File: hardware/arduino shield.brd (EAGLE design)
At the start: 100 x 54.6 mm, 26 parts, among them U1 ADS1115IDGST, U2 ARDUINO-MEGAPRO-5V, X4 MSTBA4

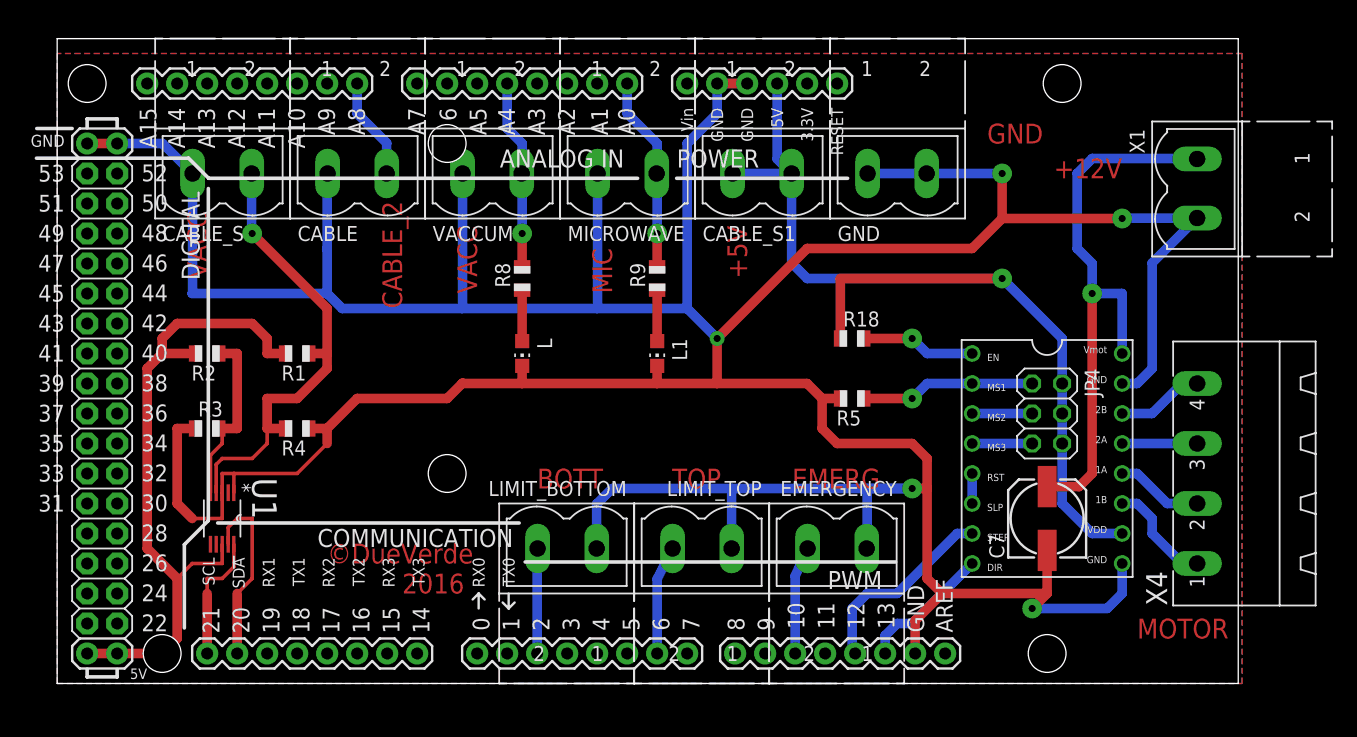
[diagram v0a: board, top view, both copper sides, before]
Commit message: hardware changes
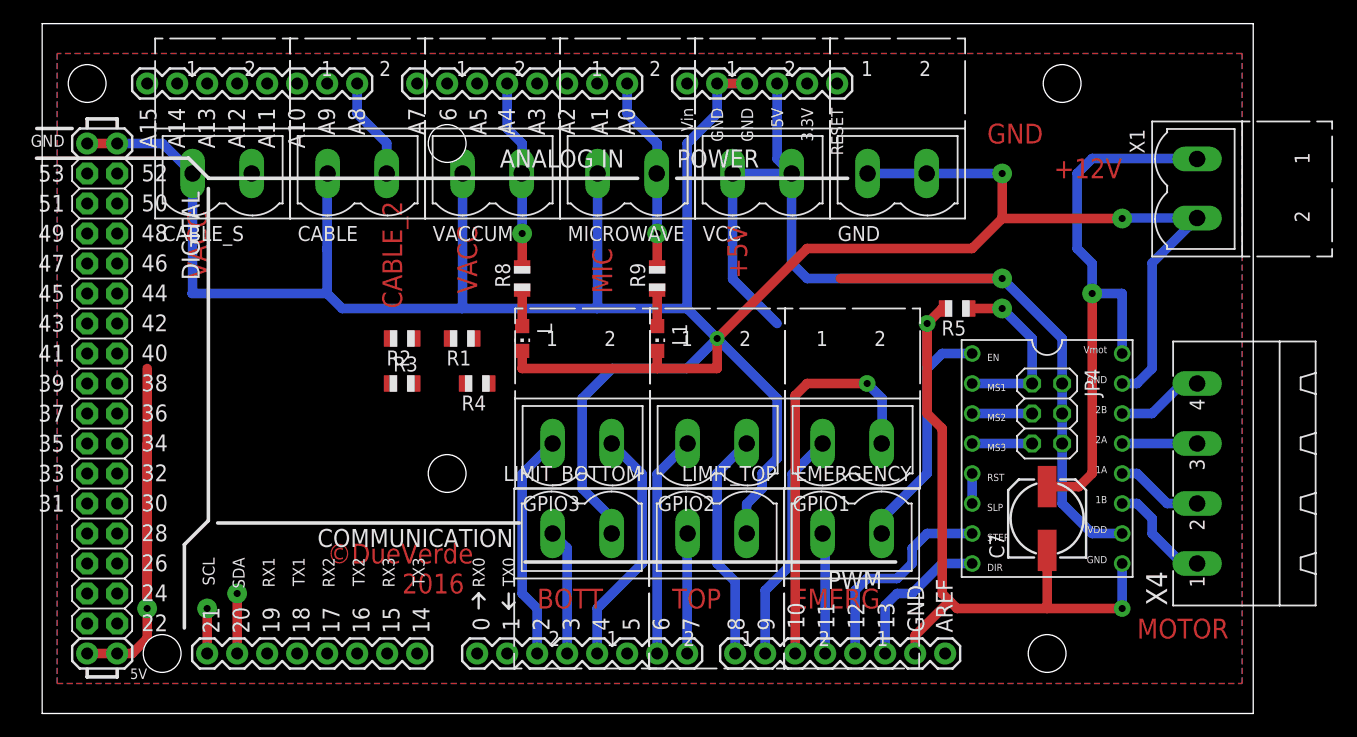
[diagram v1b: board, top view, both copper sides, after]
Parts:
- removed R18: 10k, adafruit:R0805
- removed U1: ADS1115IDGST, ADS1115:SOP50P490X110-10N
- added GPIO1, GPIO2, GPIO3: (no value), con-phoenix-500:MSTBV2
- moved R3 16.9 mm to (29.2, 25.4)
- moved R2 16.6 mm to (29.2, 29.2)
- moved R4 15.7 mm to (35.6, 25.4)
- moved R1 14.0 mm to (34.3, 29.2)
- moved R5 11.7 mm to (76.2, 31.8)
- moved LIMIT_BOTTOM 1.80 mm to (44.5, 12.7)
- moved LIMIT_TOP 1.80 mm to (55.9, 12.7)
- moved EMERGENCY 1.80 mm to (67.3, 12.7)
- moved L 1.27 mm to (39.4, 29.2)
- moved L1 1.27 mm to (50.8, 29.2)
- renumbered CABLE_S1 to VCC
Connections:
- removed net X-EN: R18.2, U$6.EN
- new net AIN0: R2.1, R3.2
- new net AIN1: CABLE_S.2, R1.1, R4.2
- new net N$5: GPIO2.2, U2.8
- new net N$8: GPIO3.1, U2.2
- new net SCL: U2.21
- new net SDA: U2.20
- net EMERGENCY: now also U2.11; no longer U2.10
- net GND: now also U$6.EN; no longer U1.1, U1.3
- net LIMIT_BOTTOM: now also U2.3; no longer U2.2
- net LIMIT_TOP: now also U2.7; no longer U2.6
- net N$3: now also GPIO1.2, U2.10; no longer U1.9, U2.20
- net N$4: now also GPIO1.1, U2.9; no longer U1.10, U2.21
- net N$6: now also GPIO2.1, U2.6; no longer R2.1, R3.2, U1.5
- net N$7: now also GPIO3.2, U2.4; no longer CABLE_S.2, R1.1, R4.2, U1.4
- net VCC: no longer R18.1, U1.8
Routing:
- net GND: track 386.5 -> 348.9 mm
- net N$5: track 0.00 -> 19.4 mm
- net N$8: track 0.00 -> 19.4 mm
- net N$7: track 39.6 -> 20.4 mm, vias 1 -> 0
- net N$3: track 15.7 -> 34.0 mm, vias 0 -> 1
- net X-EN: track 9.69 -> 0.00 mm, vias 1 -> 0
- net N$4: track 10.9 -> 19.8 mm
- net SDA: track 0.00 -> 5.08 mm, vias 0 -> 1
- net VCC: track 141.8 -> 136.8 mm, vias 1 -> 2
- net SCL: track 0.00 -> 3.81 mm, vias 0 -> 1
- net N$6: track 15.4 -> 18.8 mm
- net LIMIT_BOTTOM: track 8.89 -> 10.7 mm
- net X-DIR: track 11.4 -> 12.9 mm
- net X-STEP: track 16.7 -> 18.0 mm
- net N$2: track 4.30 -> 3.03 mm
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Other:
- board size 100 x 54.6 mm -> 102.5 x 58.4 mm
